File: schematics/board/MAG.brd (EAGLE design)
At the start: 297 x 210 mm, 12 parts

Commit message: Исправлены компоненты
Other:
- board size 297 x 210 mm -> 22 x 22 mm
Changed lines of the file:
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@@
 <board>
 <plain>
-<wire x1="0" y1="210" x2="297" y2="210" width="0.1" layer="20"/>
-<wire x1="297" y1="0" x2="297" y2="210" width="0.1" layer="20"/>
 <wire x1="10.25" y1="11.515690625" x2="10.25" y2="15.75" width="0.1" layer="20"/>
 <wire x1="16.75" y1="15.75" x2="16.75" y2="11.515690625" width="0.1" layer="20"/>

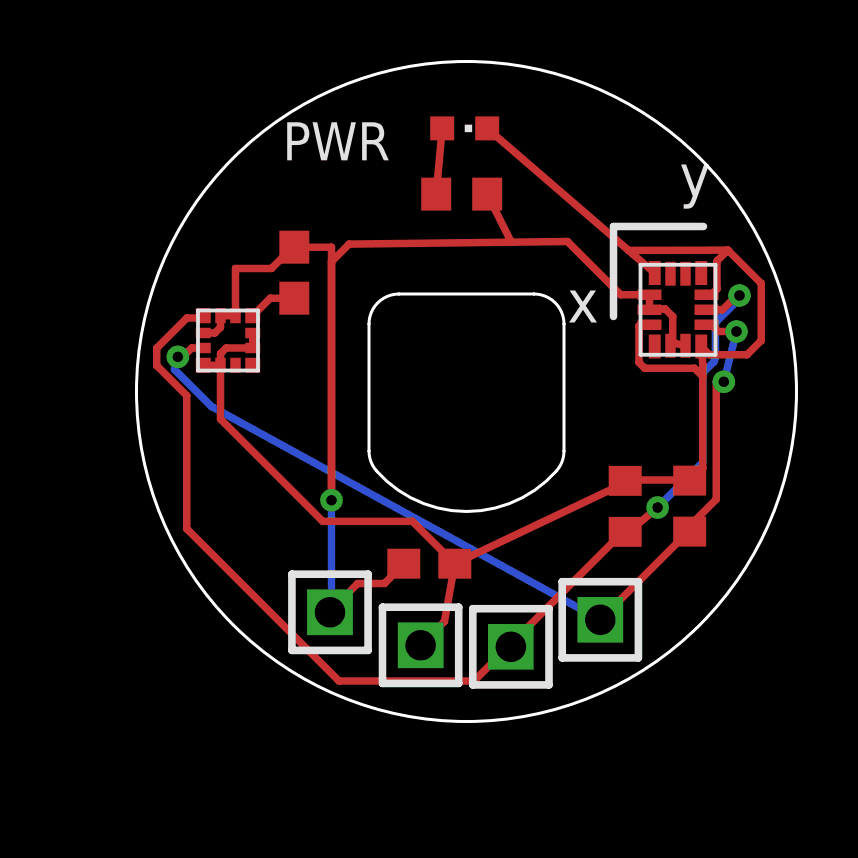
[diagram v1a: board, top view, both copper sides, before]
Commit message: Платы подготовлены для Резонита
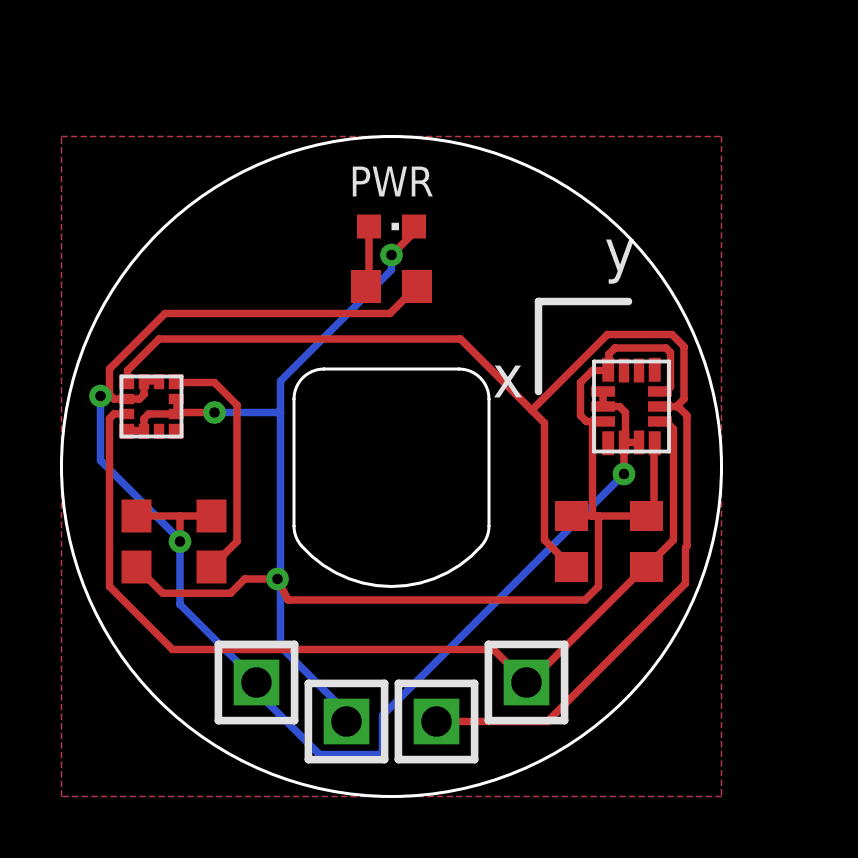
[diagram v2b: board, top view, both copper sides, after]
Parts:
- removed JP2, JP3, JP4, JP5: (no value), pinheadCS:1X01
- added 3V3, GND, SCL, SDA: (no value), pinheadCS:1X01
- moved C1 9.79 mm to (2.50, 8.50), turned to 90 degrees
- moved C10 9.38 mm to (5.00, 8.50)
- moved PWR 4.08 mm to (11.0, 19.0)
- moved R1 3.87 mm to (11.0, 17.0)
- moved LSM6DS3 3.58 mm to (19.0, 13.0)
- moved LIS3MDL 3.37 mm to (3.00, 13.0)
- moved R101 2.14 mm to (17.0, 8.50)
- moved R102 1.86 mm to (19.5, 8.50)
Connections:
- net GND: now also GND.1; no longer JP2.1
- net SCL: now also SCL.1; no longer JP5.1
- net SDA: now also SDA.1; no longer JP4.1
- net VDD: now also 3V3.1; no longer JP3.1
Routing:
- net SCL: track 38.2 -> 46.3 mm, vias 2 -> 0
- net VDD: track 52.7 -> 59.9 mm, vias 0 -> 3
- net N$3: track 1.63 -> 8.10 mm
- net GND: track 46.1 -> 51.8 mm, vias 1 -> 3
- net SDA: track 30.6 -> 32.6 mm, vias 3 -> 0
- added copper zone on layer 16, net GND
- added copper zone on layer 1, net VDD
